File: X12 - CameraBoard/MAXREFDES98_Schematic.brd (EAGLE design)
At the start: 78.9 x 14 mm, 24 parts, among them U1 MB110S-TP, U2 MB110S-TP, U3 MAX5969AETB+, U4 MAX17503ATP+

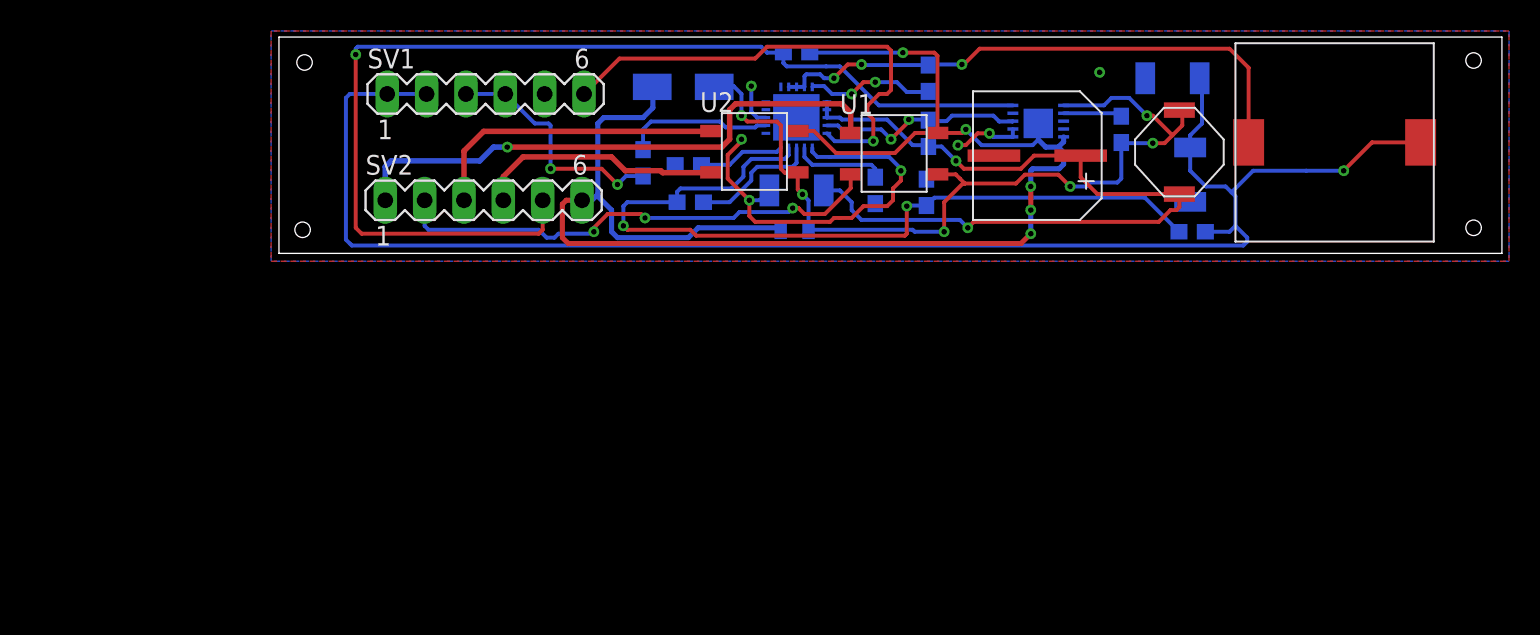
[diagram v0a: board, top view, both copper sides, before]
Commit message: rewiring
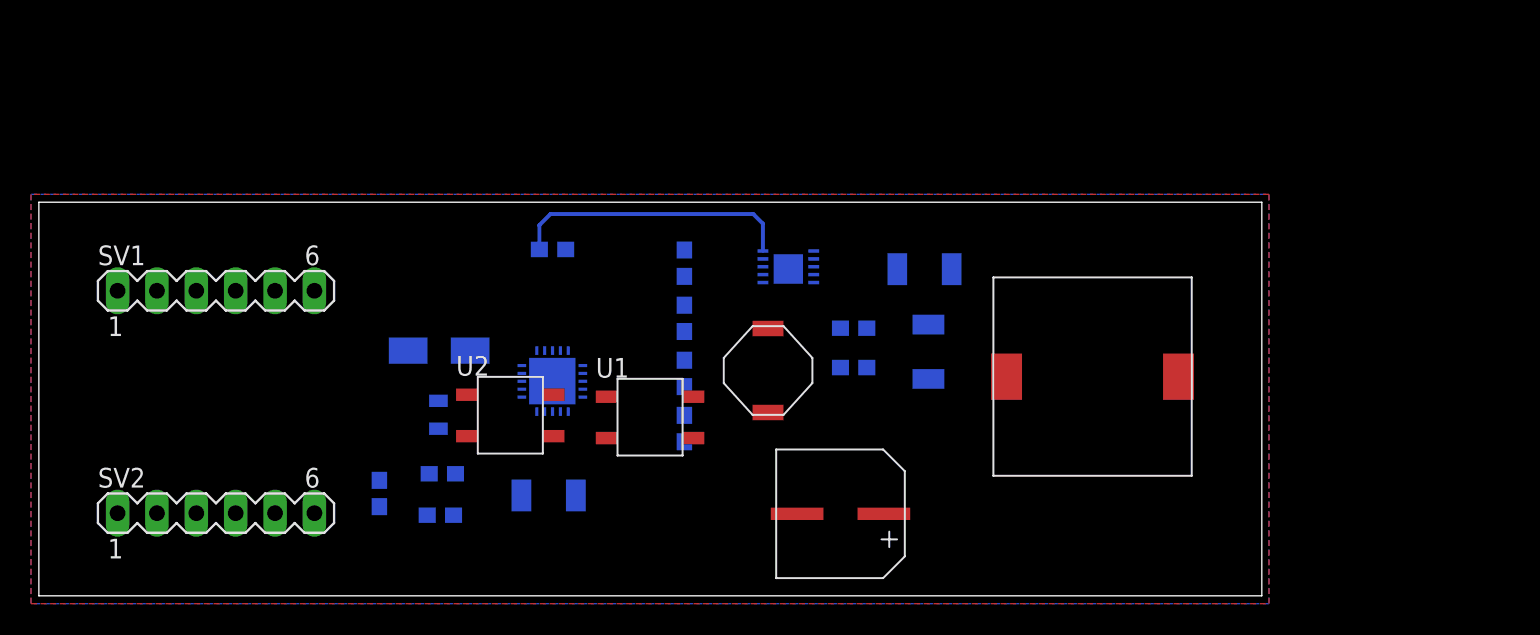
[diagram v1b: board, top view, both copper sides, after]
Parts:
- moved L1 30.1 mm to (44.2, 17.4)
- moved C8 27.3 mm to (22.0, 6.60)
- moved SV2 26.6 mm to (11.4, 5.33)
- moved C2 26.4 mm to (55.9, 1.14)
- moved C1 25.9 mm to (25.8, 11.7), turned to 90 degrees
- moved C5 25.8 mm to (25.9, 5.21)
- moved R6 25.5 mm to (26.0, 7.87)
- moved C7 25.4 mm to (32.9, 6.48)
- moved R4 23.5 mm to (52.6, 14.7)
- moved D1 23.2 mm to (29.1, 12.6)
- moved U1 23.2 mm to (35.9, 9.78)
- moved U2 23.2 mm to (26.9, 9.91)
- moved U4 23.2 mm to (35.2, 11.8)
- moved L2 21.7 mm to (61.6, 7.75)
- moved SV1 21.5 mm to (11.4, 19.7)
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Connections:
- net N$11 renamed VCC
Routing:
- net SV1_1/2: track 101.7 -> 0.00 mm, vias 1 -> 0
- net VSS_EP: track 101.0 -> 0.00 mm, vias 5 -> 0
- net VDD: track 55.6 -> 0.00 mm, vias 6 -> 0
- net FB: track 53.6 -> 0.00 mm, vias 2 -> 0
- net VIN: track 53.0 -> 0.00 mm, vias 2 -> 0
- net CLS: track 70.2 -> 18.3 mm, vias 1 -> 0
- net GND: track 49.2 -> 0.00 mm, vias 9 -> 0
- net LX: track 36.8 -> 0.00 mm, vias 3 -> 0
- net SV2_1: track 36.5 -> 0.00 mm, vias 1 -> 0
- net SV2_2: track 32.4 -> 0.00 mm, vias 3 -> 0
- net RESET: track 31.3 -> 0.00 mm, vias 1 -> 0
- net SV2_3: track 19.7 -> 0.00 mm
- net SV2_4: track 15.9 -> 0.00 mm
- net PG_EN/UVLO: track 13.3 -> 0.00 mm, vias 2 -> 0
- net VCC: track 9.66 -> 0.00 mm
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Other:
- board size 78.9 x 14 mm -> 78.9 x 25.4 mm
